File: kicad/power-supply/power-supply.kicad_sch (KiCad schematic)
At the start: 155 parts, among them J14 Conn_01x02, J15 Conn_01x02, J16 Conn_01x02, J17 Conn_01x03, J18 USB_C_Receptacle_USB2.0_16P, J3 Conn_01x02, J4 Conn_01x02, J58 Conn_01x03, J6 Conn_01x02, J8 Conn_01x02, Q1 NMOS, Q2 NMOS, Q3 NMOS, Q4 NMOS, Q5 NMOS, Q6 NMOS, Q7 NMOS, Q8 NMOS, Q9 NMOS, SW1 SW_SPST, U10 TPS568230RJER, U11 INA226, U12 TPS568230RJER, U13 TPS568230RJER, U26 HY2120, U7 HY2213-BB3A, U9 HY2213-BB3A

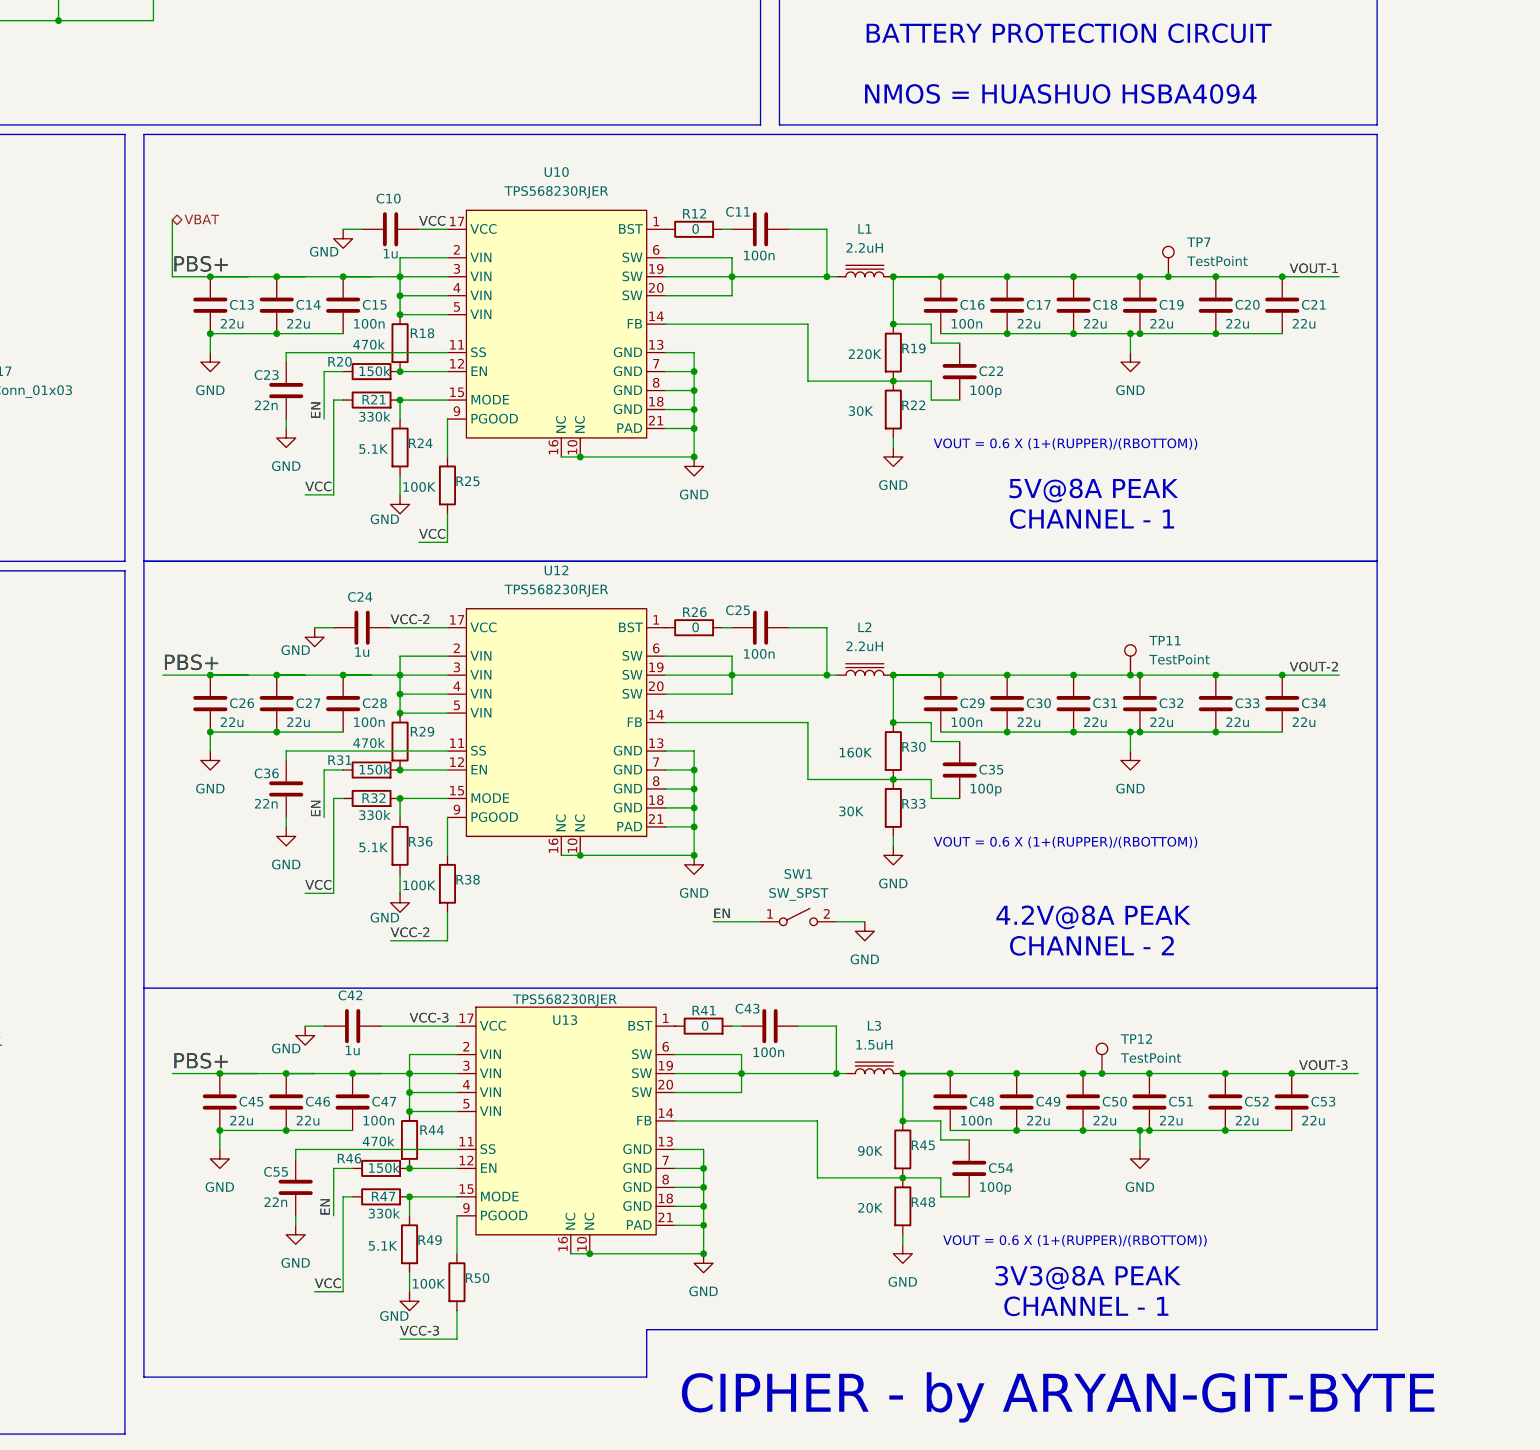
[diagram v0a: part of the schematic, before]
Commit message: changed buck converters
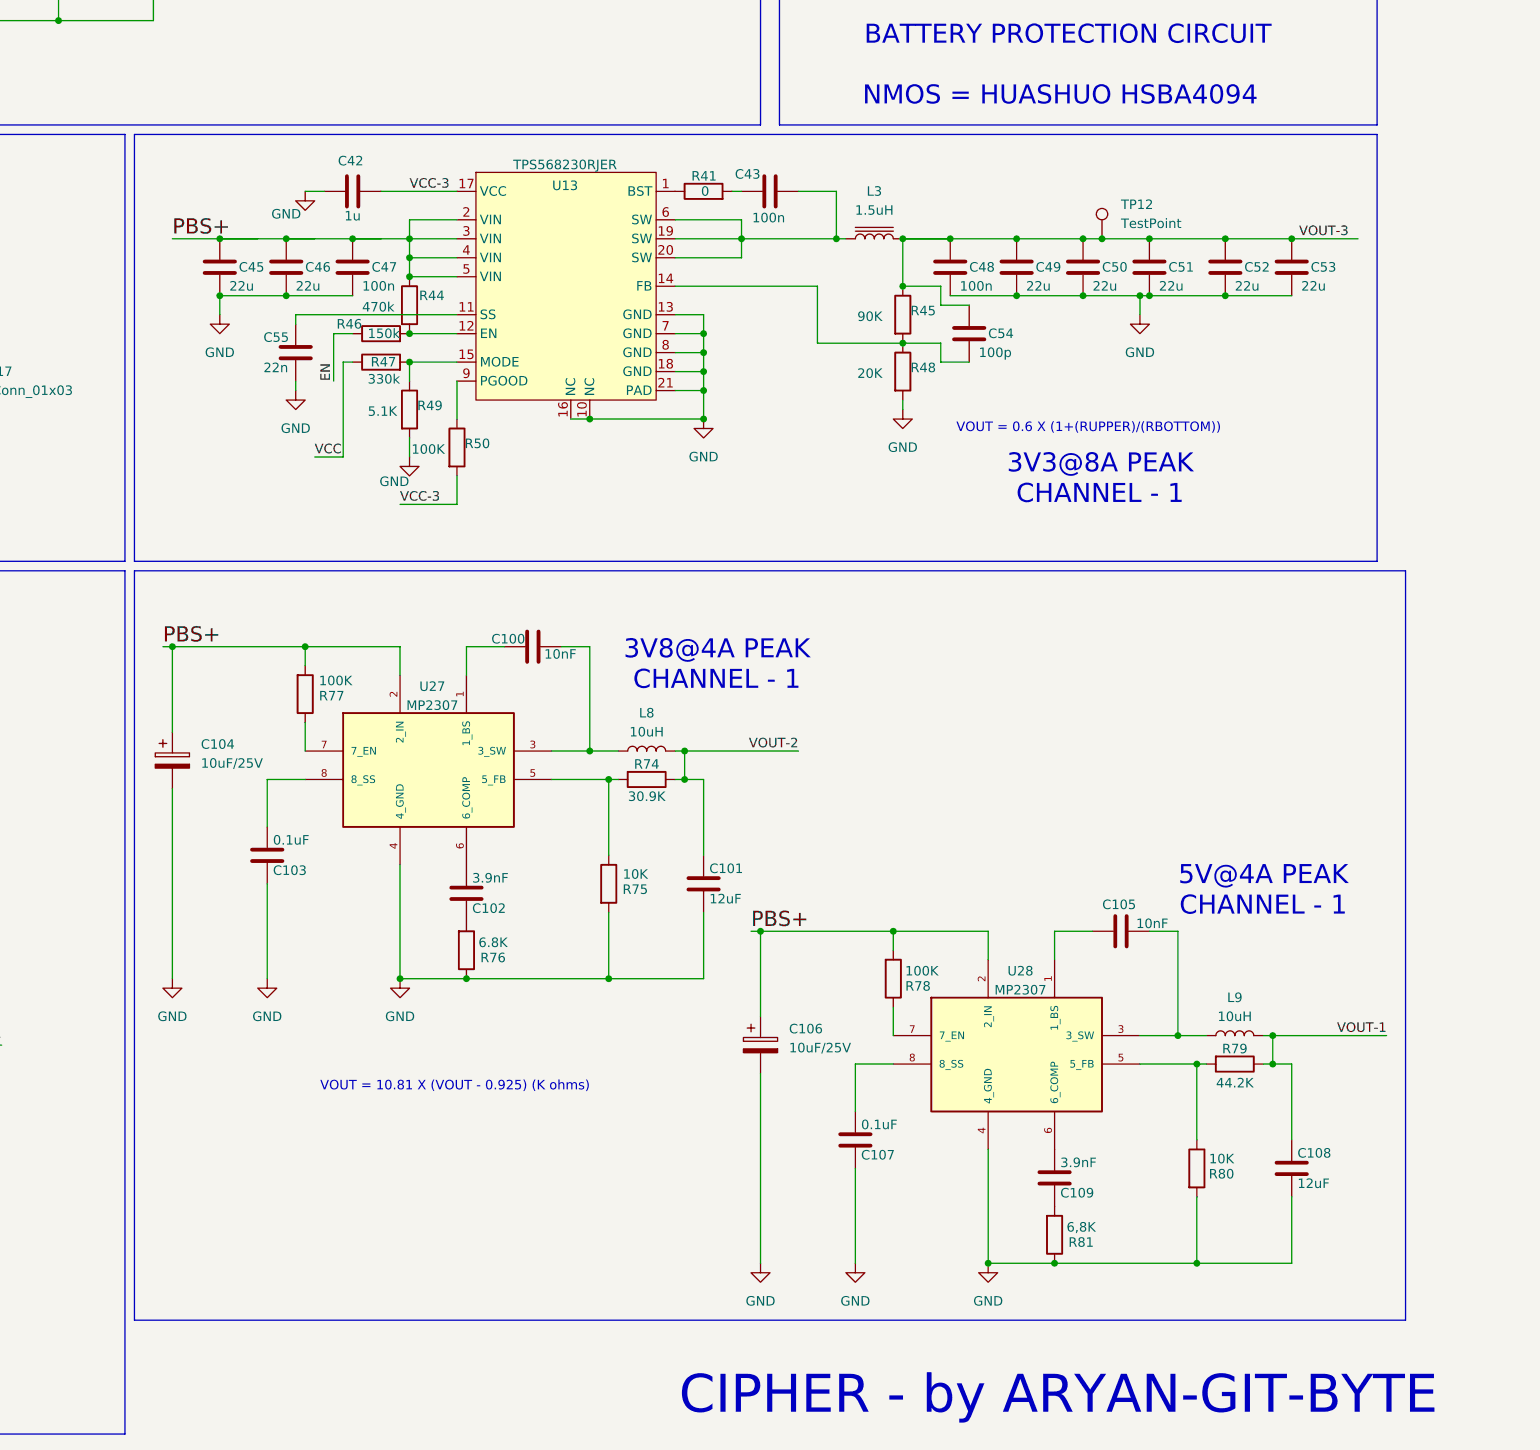
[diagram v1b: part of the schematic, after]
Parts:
- removed C10, C24: 1u, symbol Device:C
- removed C11, C15, C16, C25, C28, C29: 100n, symbol Device:C
- removed C13, C14, C17, C18, C19, C20, C21, C26, C27, C30, C31, C32, C33, C34: 22u, symbol Device:C
- removed C22, C35: 100p, symbol Device:C
- removed C23, C36: 22n, symbol Device:C
- removed L1, L2: 2.2uH, symbol Device:L_Iron
- removed R12, R26: 0, symbol Device:R
- removed R18, R29: 470k, symbol Device:R
- removed R19: 220K, symbol Device:R
- removed R20, R31: 150k, symbol Device:R
- removed R21, R32: 330k, symbol Device:R
- removed R22, R33: 30K, symbol Device:R
- removed R24, R36: 5.1K, symbol Device:R
- removed R25, R38: 100K, symbol Device:R
- removed R30: 160K, symbol Device:R
- removed SW1: SW_SPST, symbol Switch:SW_SPST
- removed TP11, TP7: TestPoint, symbol Connector:TestPoint
- removed U10, U12: TPS568230RJER, symbol TPS568230RJER:TPS568230RJER
- added C100, C105: 10nF, symbol Device:C
- added C101, C108: 12uF, symbol Device:C
- added C102, C109: 3.9nF, symbol Device:C
- added C103, C107: 0.1uF, symbol Device:C
- added C104, C106: 10uF/25V, symbol Device:C_Polarized
- added L8, L9: 10uH, symbol Device:L
- added R74: 30.9K, symbol Device:R
- added R75, R80: 10K, symbol Device:R
- added R76: 6.8K, symbol Device:R
- added R77, R78: 100K, symbol Device:R
- added R79: 44.2K, symbol Device:R
- added R81: 6,8K, symbol Device:R
- added U27, U28: MP2307, MP2307:SO-8_EP, symbol MP2307:MP2307
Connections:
- net 3V8_OUT: now also C101.1, L8.2, R74.1
- net 5V_OUT: now also C108.1, L9.2, R79.1
- net GND: now also C101.2, C103.1, C104.2, C106.2, C107.1, C108.2, R75.2, R76.1, R80.2, R81.1, U27.4 (4_GND), U28.4 (4_GND)
- net VBAT: now also C104.1, C106.1, R77.2, R78.2, U27.2 (2_IN), U28.2 (2_IN)
- new net: R78.1, U28.7 (7_EN)
- new net: C102.1, R76.2
- new net: C100.2, L8.1, U27.3 (3_SW)
- new net: C109.1, R81.2
- new net: C109.2, U28.6 (6_COMP)
- new net: C105.1, U28.1 (1_BS)
- new net: C105.2, L9.1, U28.3 (3_SW)
- new net: R79.2, R80.1, U28.5 (5_FB)
- new net: C107.2, U28.8 (8_SS)
- new net: C100.1, U27.1 (1_BS)
- new net: R74.2, R75.1, U27.5 (5_FB)
- new net: C102.2, U27.6 (6_COMP)
- new net: R77.1, U27.7 (7_EN)
- new net: C103.2, U27.8 (8_SS)
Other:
- note added: "3V8@4A PEAK CHANNEL - 1"
- note added: "5V@4A PEAK CHANNEL - 1"
- note added: "VOUT = 10.81 X (VOUT - 0.925) (K ohms)"
- note removed: "4.2V@8A PEAK CHANNEL - 2"
- note removed: "5V@8A PEAK CHANNEL - 1"
- moved on the sheet: C42, C43, C45, C46, C47, C48, C49, C50, C51, C52, C53, C54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
